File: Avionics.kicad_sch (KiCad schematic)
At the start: 49 parts, among them Q1 IRLML2803, Q10 IRF7404, Q14 IRLML2803, SW1 KMR231NG LFS, U1 MAX706RESA+, U12 DS3231M, U2 ATSAMD51J20A-AU, U3 BMX160, U6 MR25H40MDF, Y1 32.768kHz

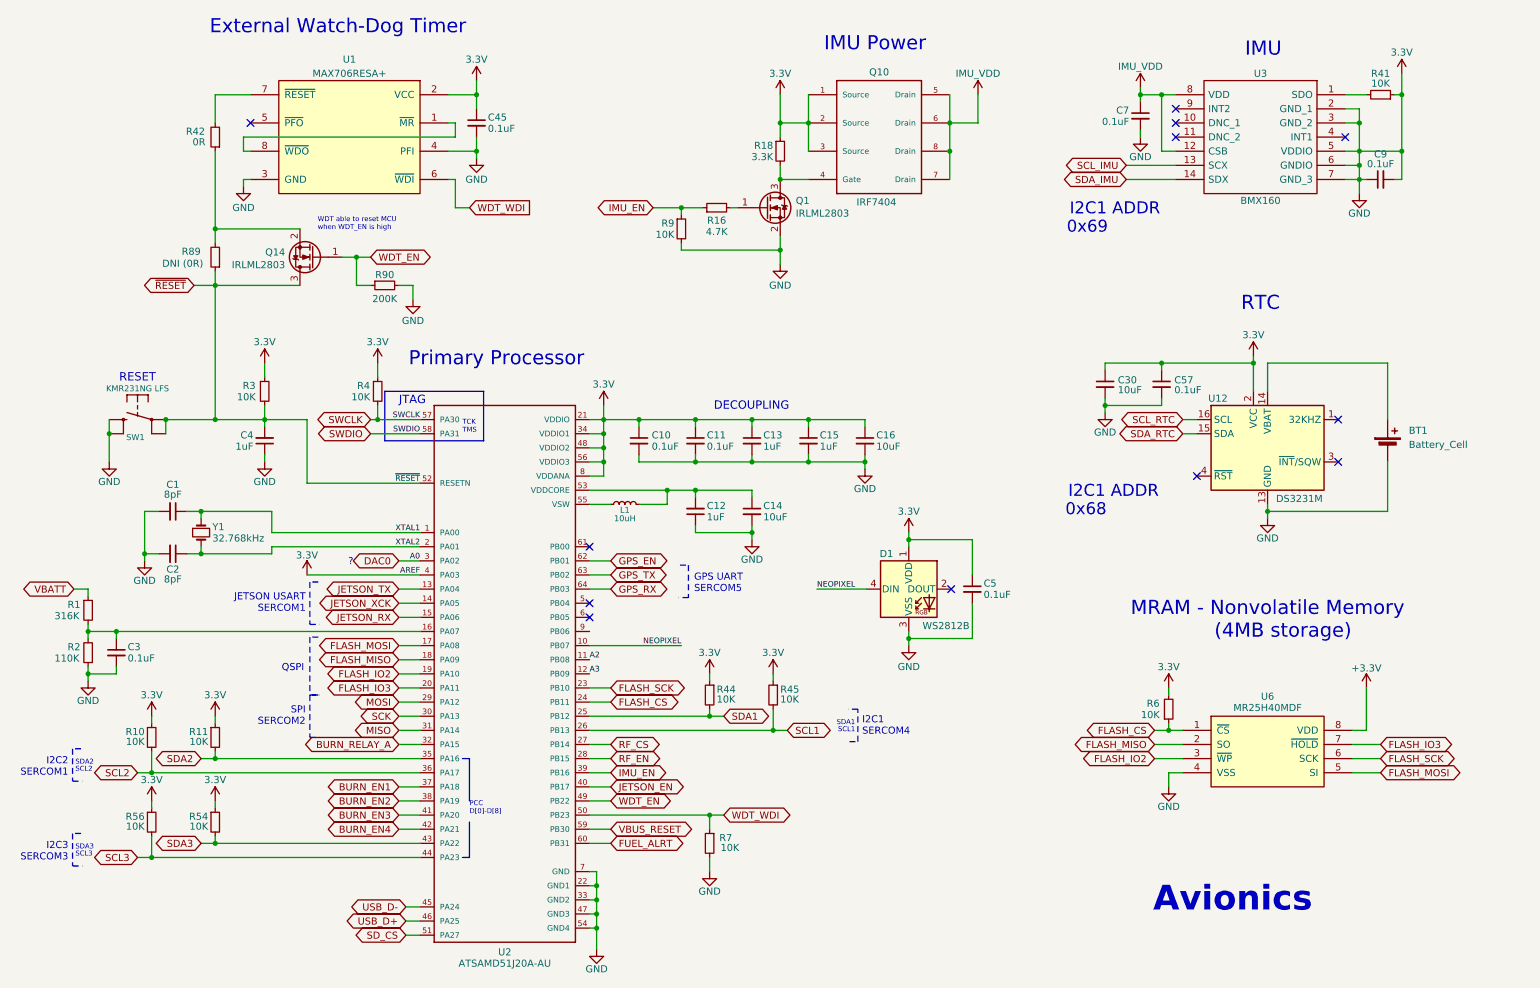
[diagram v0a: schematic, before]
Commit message: Complete layout
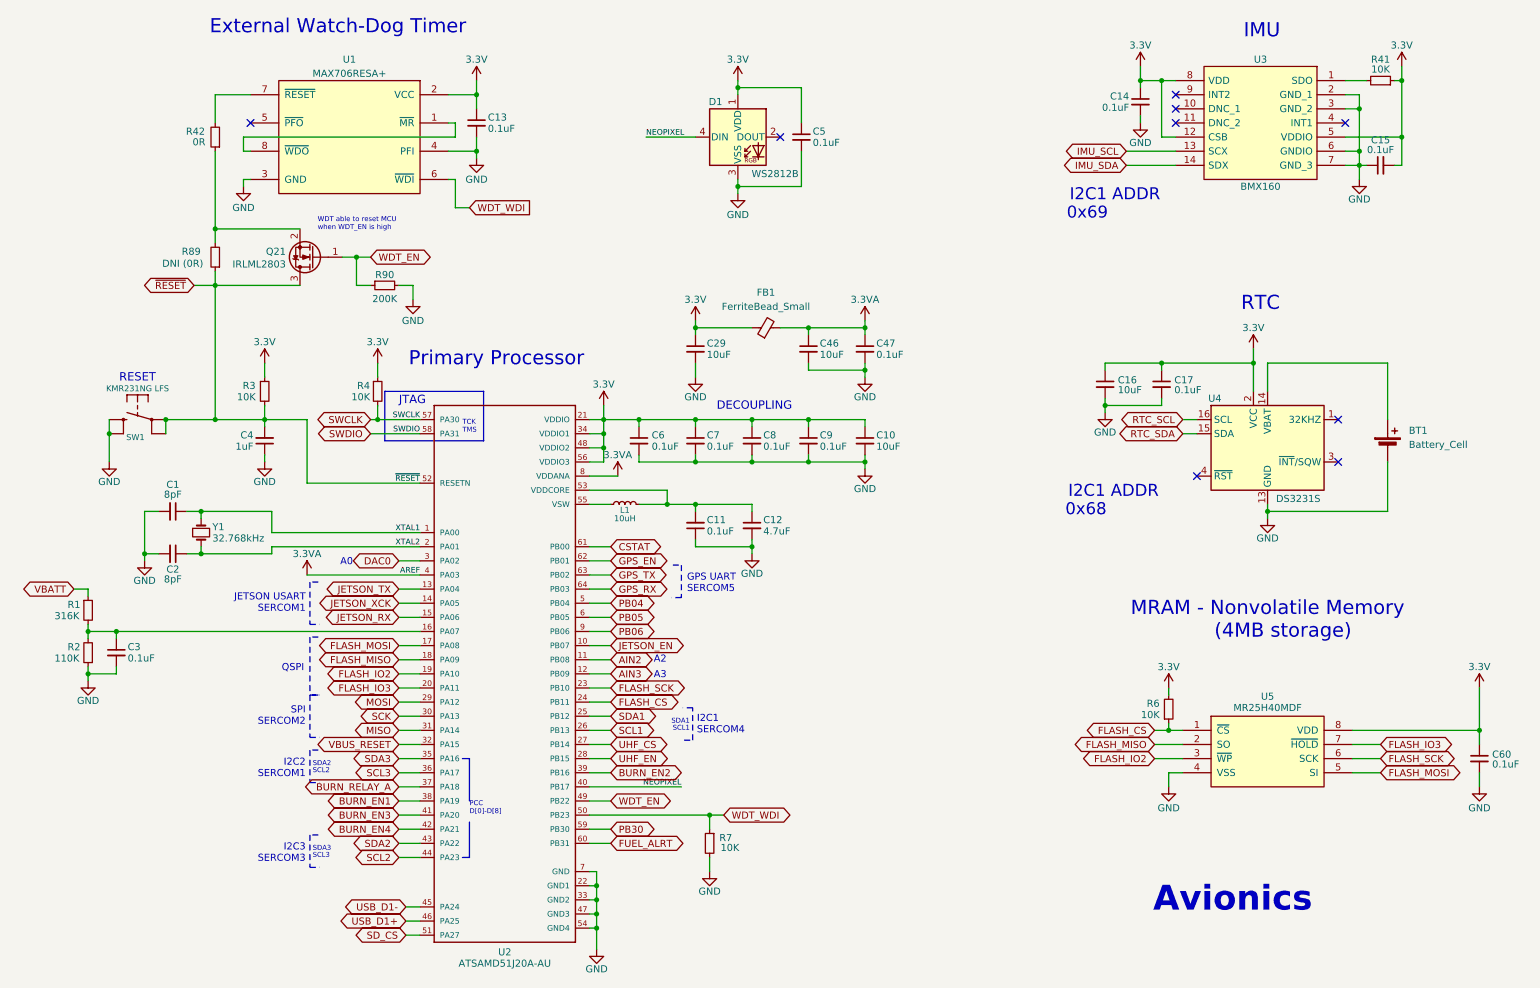
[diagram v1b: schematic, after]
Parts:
- removed Q1: IRLML2803, Package_TO_SOT_SMD:SOT-23, symbol Transistor_FET:IRLML2060
- removed Q10: IRF7404, mainboard:NDS8434, symbol mainboard:NDS8434
- removed R10, R11, R44, R45, R54, R56, R9: 10K, Resistor_SMD:R_0603_1608Metric, symbol Device:R_Small
- removed R16: 4.7K, Resistor_SMD:R_0603_1608Metric, symbol Device:R_Small
- removed R18: 3.3K, Resistor_SMD:R_0603_1608Metric, symbol Device:R_Small
- added C29, C46: 10uF, Capacitor_SMD:C_0603_1608Metric, symbol Device:C_Small
- added C47, C60: 0.1uF, Capacitor_SMD:C_0603_1608Metric, symbol Device:C_Small
- added FB1: FerriteBead_Small, Inductor_SMD:L_0603_1608Metric, symbol Device:FerriteBead_Small
- BT1: footprint (none) -> Battery:BatteryHolder_LINX_BAT-HLD-012-SMT
- C1, C2, C3, C4, C5: symbol mainboard:C_Small -> Device:C_Small
- C10: renamed from C16; symbol mainboard:C_Small -> Device:C_Small
- C11: renamed from C12; value 1uF -> 0.1uF; symbol mainboard:C_Small -> Device:C_Small
- C12: renamed from C14; value 10uF -> 4.7uF; symbol mainboard:C_Small -> Device:C_Small
- C14: renamed from C7; symbol mainboard:C_Small -> Device:C_Small
- C15: renamed from C9; symbol mainboard:C_Small -> Device:C_Small
- C16: renamed from C30; footprint (none) -> Capacitor_SMD:C_0603_1608Metric
- C17: renamed from C57; footprint (none) -> Capacitor_SMD:C_0603_1608Metric
- C6: renamed from C10; symbol mainboard:C_Small -> Device:C_Small
- C7: renamed from C11; symbol mainboard:C_Small -> Device:C_Small
- C8: renamed from C13; value 1uF -> 0.1uF; symbol mainboard:C_Small -> Device:C_Small
- C9: renamed from C15; value 1uF -> 0.1uF; symbol mainboard:C_Small -> Device:C_Small
- Q21: renamed from Q14; symbol Transistor_FET:IRLML2060 -> Mainboard:IRLML2803
- SW1: footprint mainboard:BTN_KMR2_4.6X2.8 -> Button_Switch_SMD:SW_Push_1P1T_NO_CK_KMR2; symbol mainboard:SWITCH_SMT4.6X2.8 -> Mainboard:KMR231
- U1: symbol mainboard:MAX708RESA+ -> Mainboard:MAX706RESA+
- U2: footprint mainboard:QFP50P1200X1200X120-64N -> Package_QFP:TQFP-64_10x10mm_P0.5mm; symbol mainboard:ATSAMD51J20A-AU-ATSAMD51J20A-AU-lab64_SAM32-rescue-lab64_SAM32-rescue-SAMD-10-rescue-SAM32-rescue -> Mainboard:ATSAMD51J20A; Flight ATSAMD51J19A-AU -> ATSAMD51J20A-AU; Manufacturer_Part_Number ATSAMD51J19A-AU -> ATSAMD51J20A-AU; Proto ATSAMD51J19A-AU -> ATSAMD51J20A-AU
- U3: footprint mainboard:BMX160 -> Package_LGA:Bosch_LGA-14_3x2.5mm_P0.5mm; symbol mainboard:BMX160 -> Mainboard:BMX160
- U4: renamed from U12; value DS3231M -> DS3231S
- U5: renamed from U6; footprint (none) -> Package_DFN_QFN:DFN-8-1EP_6x5mm_P1.27mm_EP2x2mm; symbol mainboard:MR25H40MDF -> Mainboard:MR25H40MDF
- renumbered C45 to C13
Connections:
- net +3.3V is gone; now on net 3.3V: U5.8 (VDD)
- net IMU_EN is gone; now on net BURN_EN2: U2.39 (PB16)
- net IMU_VDD is gone; now on net 3.3V: C14.1, U3.12 (CSB), U3.8 (VDD)
- net 3.3V: now also C29.1, C60.1, FB1.1; no longer BT1.2 (-), C1.2, C10.2, C11.1, C12.2, C13.2, C14.2, C15.1, C16.2, C17.2, C2.2, C3.2, C4.1, C5.2, C6.2, C7.2, C8.2, C9.2, D1.3 (VSS), R2.1, R7.2, R90.2, SW1.B (S), SW1.B' (S1), U1.3 (GND), U1.4 (PFI), U2.22 (GND1), U2.33 (GND2), U2.4 (PA03), U2.47 (GND3), U2.54 (GND4), U2.7 (GND), U2.8 (VDDANA), U3.2 (GND_1), U3.3 (GND_2), U3.6 (GNDIO), U3.7 (GND_3), U4.10 (GND), U4.11 (GND), U4.12 (GND), U4.13 (GND), U4.5 (GND), U4.6 (GND), U4.7 (GND), U4.8 (GND), U4.9 (GND), U5.4 (VSS), U5.9 (EP)
- net BURN_EN1: now also U2.38 (PA19); no longer U2.37 (PA18)
- net BURN_EN2: no longer U2.38 (PA19)
- net BURN_RELAY_A: now also U2.37 (PA18); no longer U2.32 (PA15)
- net JETSON_EN: now also U2.10 (PB07); no longer U2.40 (PB17)
- net NEOPIXEL: now also U2.40 (PB17); no longer U2.10 (PB07)
- net SCL2: now also U2.44 (PA23); no longer U2.36 (PA17)
- net SCL3: now also U2.36 (PA17); no longer U2.44 (PA23)
- net SDA2: now also U2.43 (PA22); no longer U2.35 (PA16)
- net SDA3: now also U2.35 (PA16); no longer U2.43 (PA22)
- net VBUS_RESET: now also U2.32 (PA15); no longer U2.59 (PB30)
- net ~{RESET}: now also SW1.1 (P1); no longer SW1.A (P), SW1.A' (P1)
- net PB04: now reaches U2.5 (PB04)
- net PB05: now reaches U2.6 (PB05)
- net CSTAT: now reaches U2.61 (PB00)
- net PB06: now reaches U2.9 (PB06)
- net A2 renamed AIN2
- net A3 renamed AIN3
- net RF_CS renamed UHF_CS
- net RF_EN renamed UHF_EN
- net SCL_IMU renamed IMU_SCL
- net SCL_RTC renamed RTC_SCL
- net SDA_IMU renamed IMU_SDA
- net SDA_RTC renamed RTC_SDA
- net USB_D+ renamed USB_D1+
- net USB_D- renamed USB_D1-
- new net 3.3VA: C46.1, C47.1, FB1.2, U2.4 (PA03), U2.8 (VDDANA)
- new net GND: BT1.2 (-), C1.2, C10.2, C11.1, C12.2, C13.2, C14.2, C15.1, C16.2, C17.2, C2.2, C29.2, C3.2, C4.1, C46.2, C47.2, C5.2, C6.2, C60.2, C7.2, C8.2, C9.2, D1.3 (VSS), R2.1, R7.2, R90.2, SW1.2 (S1), U1.3 (GND), U1.4 (PFI), U2.22 (GND1), U2.33 (GND2), U2.47 (GND3), U2.54 (GND4), U2.7 (GND), U3.2 (GND_1), U3.3 (GND_2), U3.6 (GNDIO), U3.7 (GND_3), U4.10 (GND), U4.11 (GND), U4.12 (GND), U4.13 (GND), U4.5 (GND), U4.6 (GND), U4.7 (GND), U4.8 (GND), U4.9 (GND), U5.4 (VSS), U5.9 (EP)
- new net PB30: U2.59 (PB30)
- no-connect marks 12 -> 9
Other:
- note added: "A0"
- note added: "A2"
- note added: "A3"
- note removed: "?"
- note removed: "IMU Power"
- moved on the sheet: C11, C12, C14, C15, C5, D1, R41

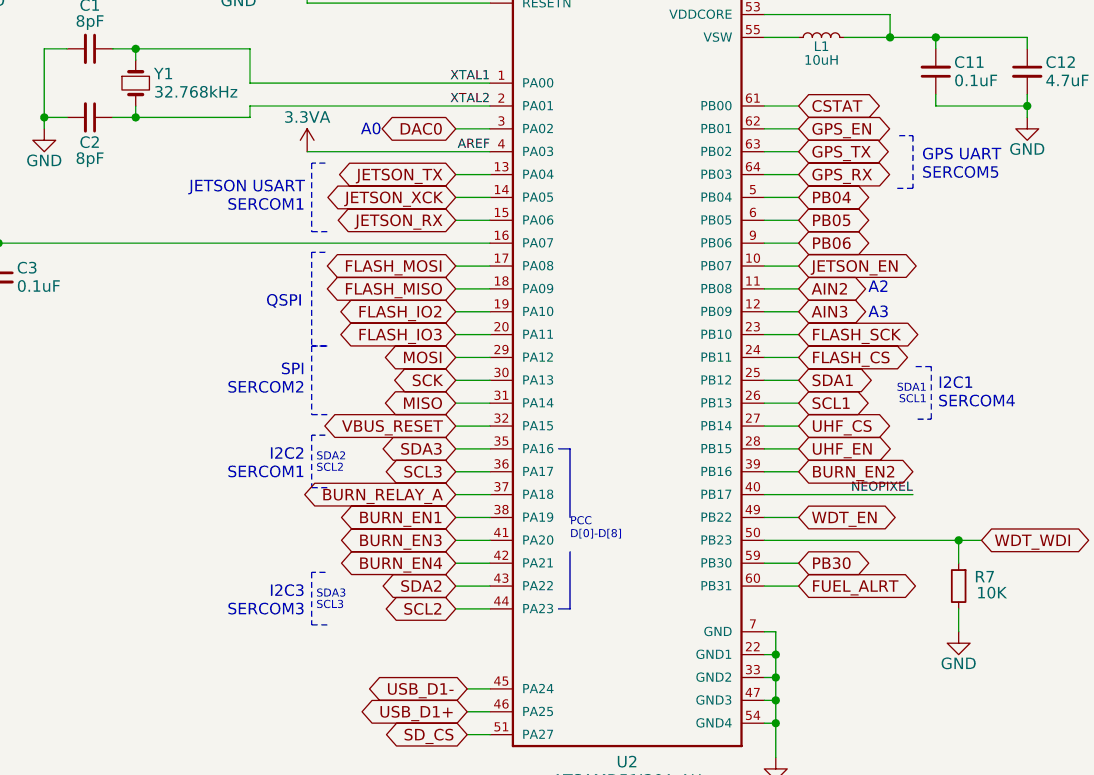
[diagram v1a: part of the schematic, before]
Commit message: v1 Final
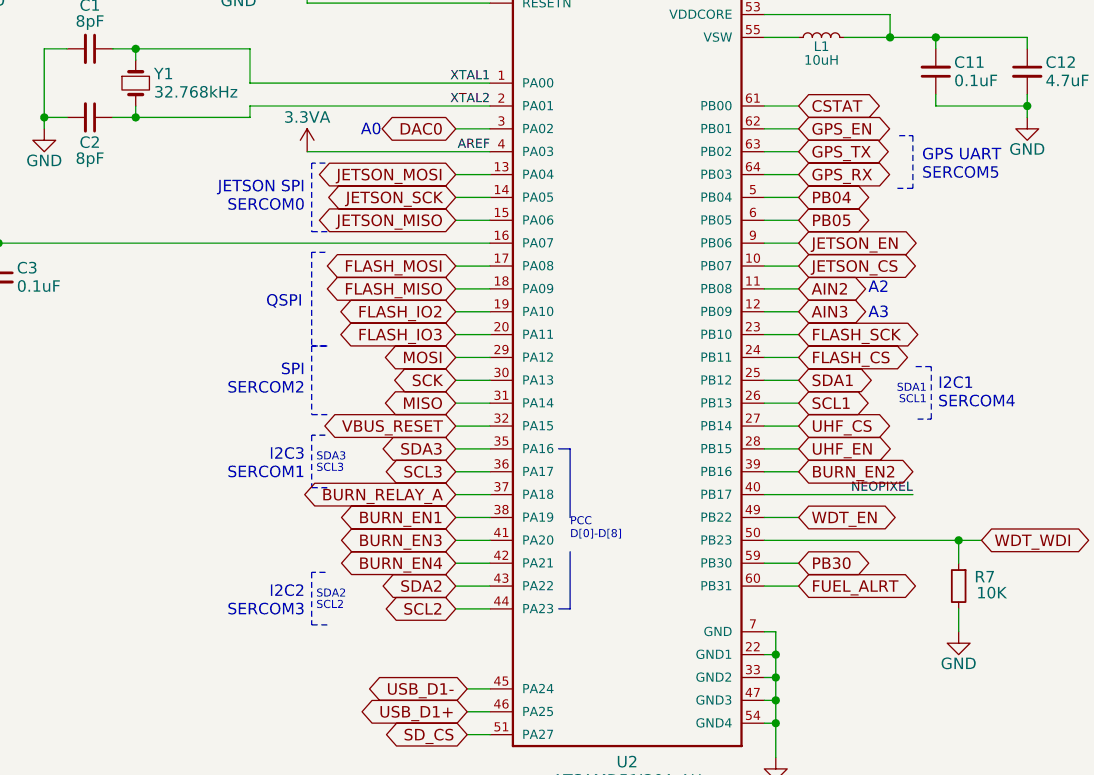
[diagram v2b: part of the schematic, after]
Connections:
- net PB06 is gone; now on net JETSON_EN: U2.9 (PB06)
- net JETSON_EN: no longer U2.10 (PB07)
- net JETSON_RX renamed JETSON_MISO
- net JETSON_TX renamed JETSON_MOSI
- net JETSON_XCK renamed JETSON_SCK
- new net JETSON_CS: U2.10 (PB07)
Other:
- note added: "I2C2 SERCOM3"
- note added: "I2C3 SERCOM1"
- note added: "JETSON SPI SERCOM0"
- note removed: "I2C2 SERCOM1"
- note removed: "I2C3 SERCOM3"
- note removed: "JETSON USART SERCOM1"
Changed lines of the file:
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@@
 	(wire
 		(pts
+			(xy 81.28 120.65) (xy 85.09 120.65)
+		)
+		(stroke
+			(width 0)
+			(type default)
+		)
+	)
+	(wire
+		(pts
 			(xy 77.47 77.47) (xy 77.47 80.01)
 		)
@@
 		)
 	)
+	(wire
+		(pts
+			(xy 81.28 118.11) (xy 85.09 118.11)
+		)
+		(stroke
+			(width 0)
+			(type default)
+		)
+	)
 	(polyline
 		(pts
@@
 	(wire
 		(pts
-			(xy 81.28 123.19) (xy 85.09 123.19)
-		)
-		(stroke
-			(width 0)
-			(type default)
-		)
-	)
-	(wire
-		(pts
 			(xy 64.77 115.57) (xy 85.09 115.57)
 		)
@@
 	(wire
 		(pts
-			(xy 81.28 120.65) (xy 85.09 120.65)
+			(xy 254 29.21) (xy 254 31.75)
 		)
 		(stroke
@@
 	(wire
 		(pts
-			(xy 254 29.21) (xy 254 31.75)
+			(xy 137.16 166.37) (xy 137.16 168.91)
 		)
 		(stroke
@@
 	(wire
 		(pts
-			(xy 137.16 166.37) (xy 137.16 168.91)
+			(xy 30.48 125.73) (xy 85.09 125.73)
 		)
 		(stroke
@@
 	(wire
 		(pts
-			(xy 30.48 125.73) (xy 85.09 125.73)
+			(xy 81.28 123.19) (xy 85.09 123.19)
 		)
 		(stroke
@@
 	(wire
 		(pts
-			(xy 81.28 118.11) (xy 85.09 118.11)
-		)
-		(stroke
-			(width 0)
-			(type default)
-		)
-	)
-	(wire
-		(pts
 			(xy 208.28 78.74) (xy 208.28 77.47)
 		)
@@
 		)
 	)
-	(text "SDA2"
+	(text "SDA3"
 		(exclude_from_sim no)
 		(at 65.786 150.114 0)
@@
 		)
 	)
-	(text "I2C2\nSERCOM1"
+	(text "I2C3\nSERCOM1"
 		(exclude_from_sim no)
 		(at 64.516 150.368 0)
@@
 		)
 	)
-	(text "SDA3"
+	(text "SDA2"
 		(exclude_from_sim no)
 		(at 65.786 165.354 0)
@@
 		)
 	)
-	(text "SCL3"
+	(text "SCL2"
 		(exclude_from_sim no)
 		(at 65.786 166.624 0)
@@
 		)
 	)
-	(text "SCL2"
+	(text "SCL3"
 		(exclude_from_sim no)
 		(at 65.786 151.384 0)
@@
 		)
 	)
-	(text "JETSON USART\nSERCOM1"
+	(text "JETSON SPI\nSERCOM0"
 		(exclude_from_sim no)
 		(at 64.516 120.65 0)
@@
 		)
 	)
-	(text "I2C3\nSERCOM3"
+	(text "I2C2\nSERCOM3"
 		(exclude_from_sim no)
 		(at 64.516 165.608 0)
@@
 		)
 	)
-	(global_label "JETSON_TX"
-		(shape bidirectional)
-		(at 81.28 118.11 180)
-		(effects
-			(font
-				(size 1.27 1.27)
-			)
-			(justify right)
-		)
-		(property "Intersheetrefs" "${INTERSHEET_REFS}"
-			(at 81.28 118.11 0)
-			(effects
-				(font
-					(size 1.27 1.27)
-				)
-				(hide yes)
-			)
-		)
-	)
-	(global_label "JETSON_XCK"
+	(global_label "JETSON_SCK"
 		(shape bidirectional)
 		(at 81.28 120.65 180)
@@
 		)
 	)
-	(global_label "PB06"
+	(global_label "JETSON_CS"
 		(shape bidirectional)
-		(at 119.38 125.73 0)
+		(at 119.38 128.27 0)
 		(fields_autoplaced yes)
 		(effects
@@
 		)
 		(property "Intersheetrefs" "${INTERSHEET_REFS}"
-			(at 127.6225 125.73 0)
+			(at 133.0653 128.27 0)
 			(effects
 				(font
@@
 		)
 	)
+	(global_label "JETSON_MISO"
+		(shape bidirectional)
+		(at 81.28 123.19 180)
+		(effects
+			(font
+				(size 1.27 1.27)
+			)
+			(justify right)
+		)
+		(property "Intersheetrefs" "${INTERSHEET_REFS}"
+			(at 81.28 123.19 0)
+			(effects
+				(font
+					(size 1.27 1.27)
+				)
+				(hide yes)
+			)
+		)
+	)
 	(global_label "SDA1"
 		(shape bidirectional)
@@
 		)
 	)
+	(global_label "JETSON_MOSI"
+		(shape bidirectional)
+		(at 81.28 118.11 180)
+		(effects
+			(font
+				(size 1.27 1.27)
+			)
+			(justify right)
+		)
+		(property "Intersheetrefs" "${INTERSHEET_REFS}"
+			(at 81.28 118.11 0)
+			(effects
+				(font
+					(size 1.27 1.27)
+				)
+				(hide yes)
+			)
+		)
+	)
 	(global_label "PB04"
 		(shape bidirectional)
@@
 		)
 	)
-	(global_label "JETSON_RX"
-		(shape bidirectional)
-		(at 81.28 123.19 180)
-		(effects
-			(font
-				(size 1.27 1.27)
-			)
-			(justify right)
-		)
-		(property "Intersheetrefs" "${INTERSHEET_REFS}"
-			(at 81.28 123.19 0)
-			(effects
-				(font
-					(size 1.27 1.27)
-				)
-				(hide yes)
-			)
-		)
-	)
 	(global_label "PB05"
 		(shape bidirectional)
@@
 	(global_label "JETSON_EN"
 		(shape bidirectional)
-		(at 119.38 128.27 0)
+		(at 119.38 125.73 0)
 		(effects
 			(font
@@
 		)
 		(property "Intersheetrefs" "${INTERSHEET_REFS}"
-			(at 119.38 128.27 0)
+			(at 119.38 125.73 0)
 			(effects
 				(font
